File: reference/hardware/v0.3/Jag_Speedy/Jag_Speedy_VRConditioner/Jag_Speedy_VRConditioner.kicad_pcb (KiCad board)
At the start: 2 copper layers, 36.8 x 27.9 mm, 15 parts, among them IC1 MAX9926UAEE+, J1 Conn

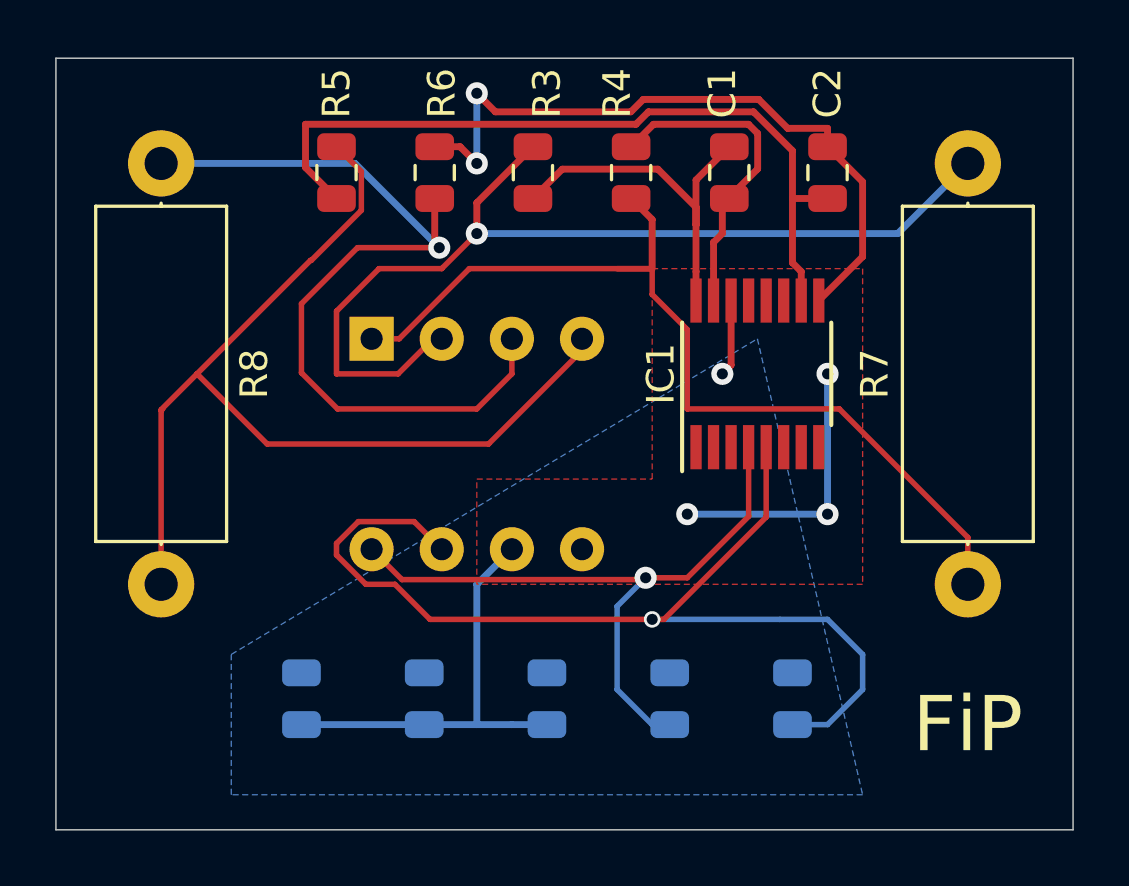
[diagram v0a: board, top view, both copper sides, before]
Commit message: PCB Changes
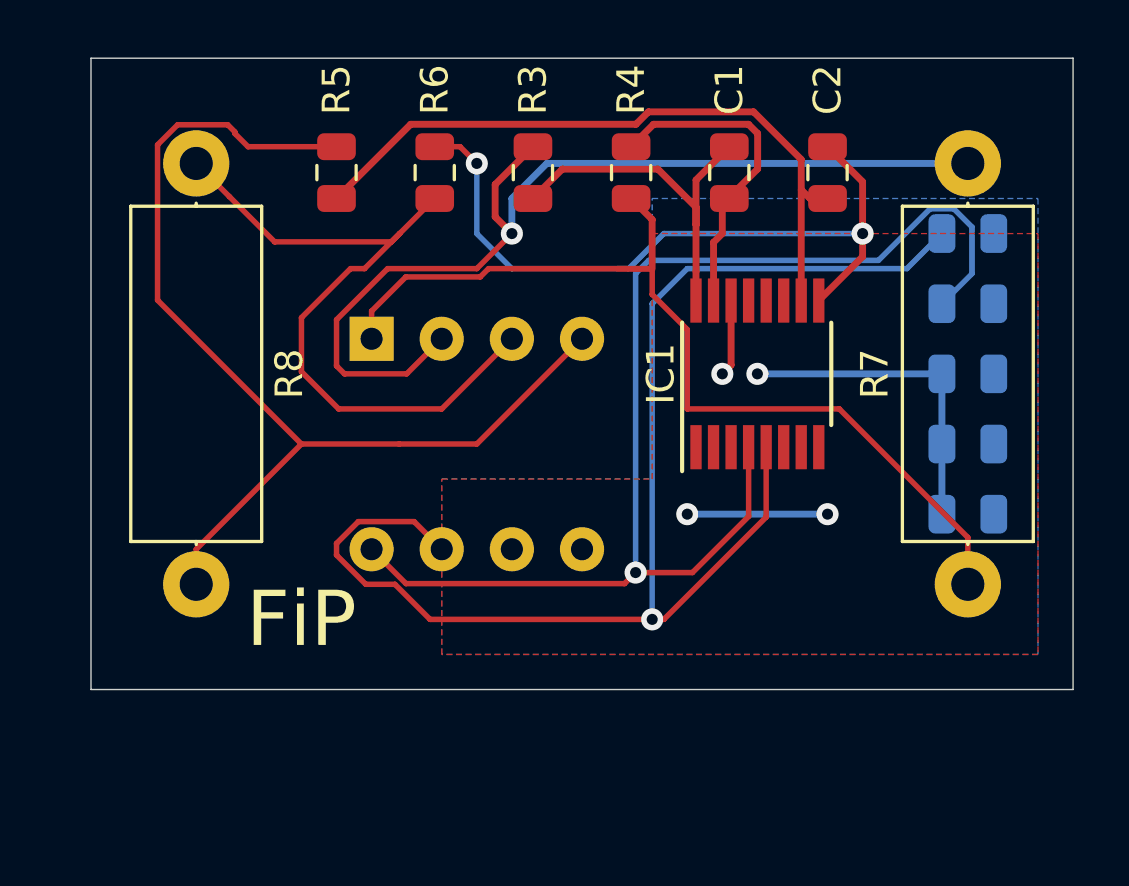
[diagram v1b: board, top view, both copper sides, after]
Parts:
- moved C5 25.0 mm to (156.2, 95.2), turned to 180 degrees
- moved C4 21.7 mm to (156.2, 92.7), turned to 180 degrees
- moved C3 19.3 mm to (156.2, 90.2), turned to 180 degrees
- moved R2 18.0 mm to (156.2, 85.1), turned to 0 degrees
- moved R1 17.9 mm to (156.2, 87.6), turned to 0 degrees
- moved R8 1.27 mm to (128.3, 82.5)
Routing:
- net Output1: track 24.5 -> 45.2 mm
- net Output2: track 38.0 -> 48.5 mm
- net Ground: track 25.9 -> 16.8 mm
- net VR2+: track 31.5 -> 26.5 mm, vias 1 -> 0
- net Net-(C2-Pad1): track 28.4 -> 25.0 mm
- net VR2-: track 36.2 -> 38.5 mm
- net Net-(C2-Pad2): track 25.3 -> 26.1 mm
- net VR1-: track 34.7 -> 35.3 mm
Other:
- board size 36.8 x 27.9 mm -> 35.6 x 22.9 mm
